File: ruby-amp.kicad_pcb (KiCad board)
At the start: 2 copper layers, 23 parts, among them J1 AudioJack3_Switch, J2 AudioJack2_Dual_Ground_Switch, P1 10k, P2 100K, P3 1k Lin, Q1 MPF102_DSG, U1 LM386

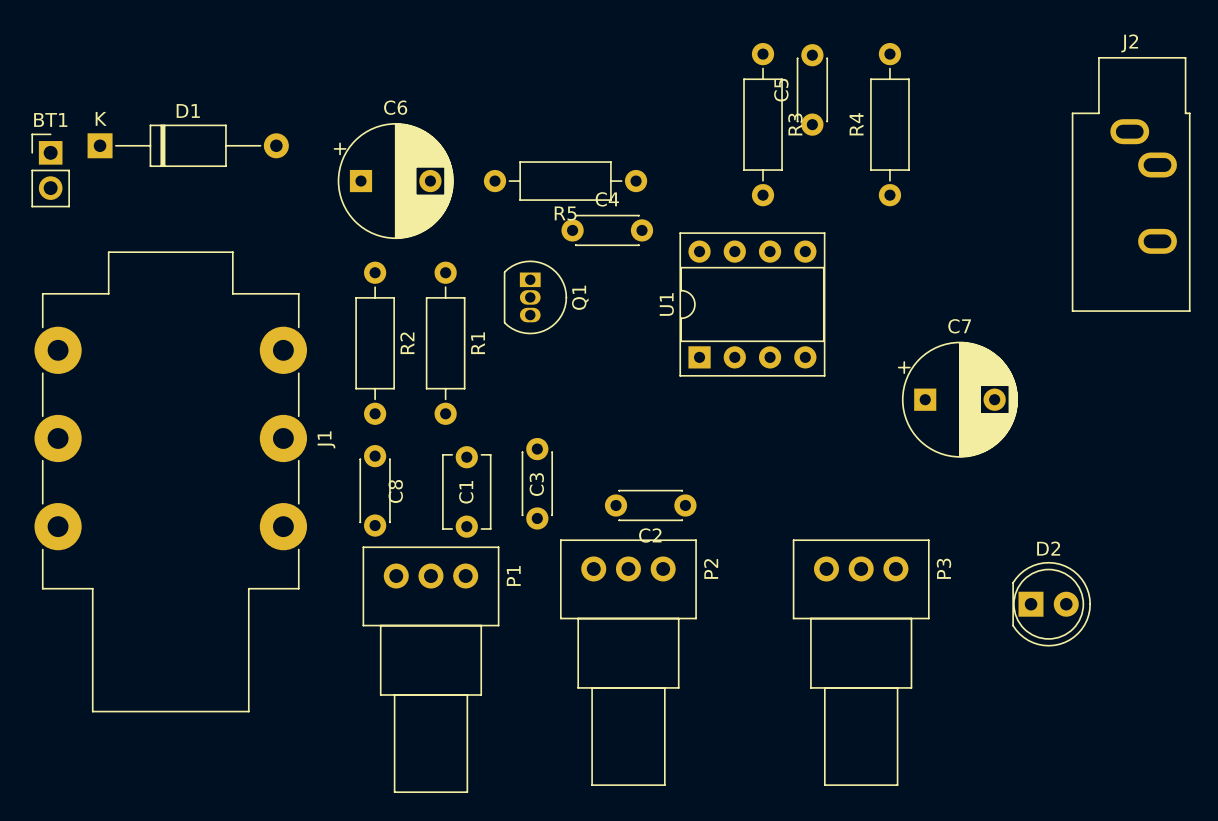
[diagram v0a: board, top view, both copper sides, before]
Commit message: PCB primera iteración
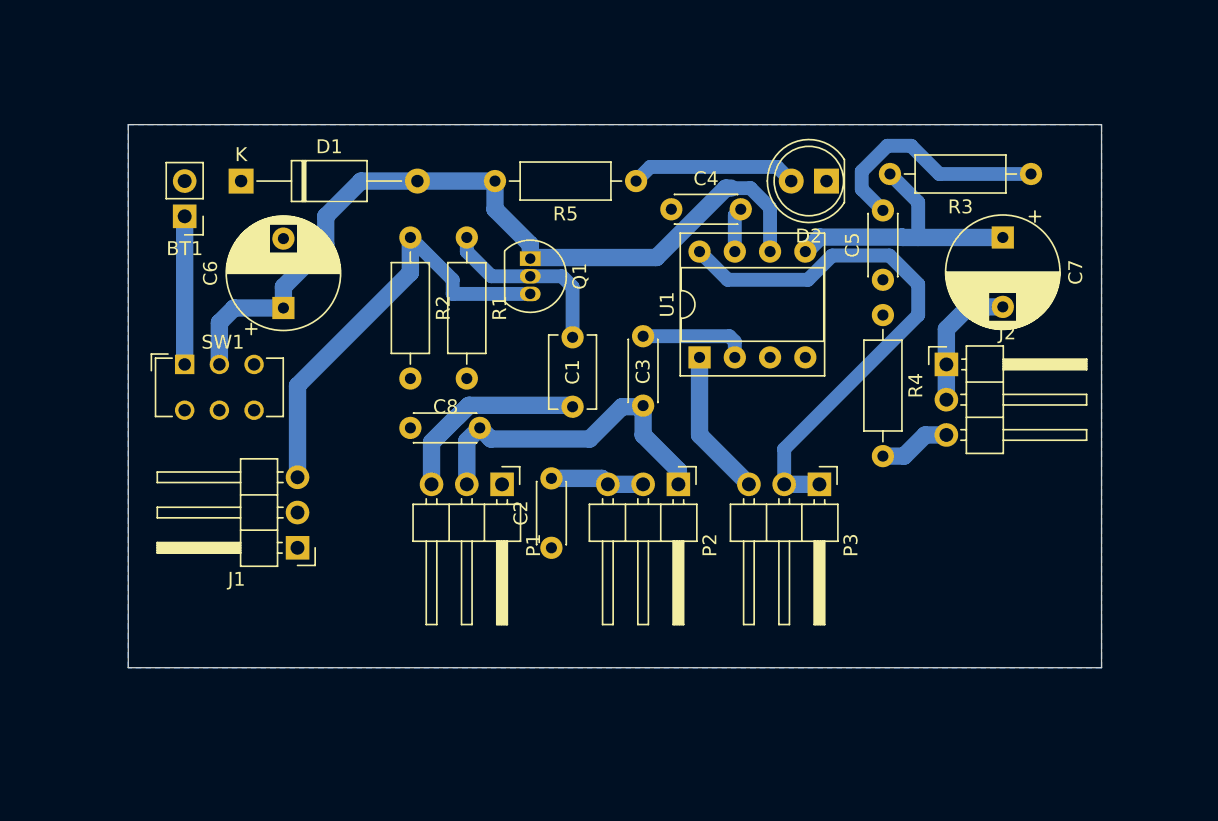
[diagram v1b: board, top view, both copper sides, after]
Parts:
- added SW1: SW_DPDT_x2, Button_Switch_THT:SW_CuK_JS202011CQN_DPDT_Straight, F.Cu at (111.3, 79.2)
- J1: value AudioJack3_Switch -> Input_Signal; footprint Connector_Audio:Jack_6.35mm_Neutrik_NMJ6HFD4_Horizontal -> Connector_PinHeader_2.54mm:PinHeader_1x03_P2.54mm_Horizontal
- J2: value AudioJack2_Dual_Ground_Switch -> Output_Signal; footprint Connector_Audio:Jack_3.5mm_CUI_SJ1-3533NG_Horizontal -> Connector_PinHeader_2.54mm:PinHeader_1x03_P2.54mm_Horizontal
- P1, P2, P3: footprint Potentiometer_THT:Potentiometer_Alps_RK09Y11_Single_Horizontal -> Connector_PinHeader_2.54mm:PinHeader_1x03_P2.54mm_Horizontal
- moved D2 33.9 mm to (157.5, 66.0), turned to 180 degrees
- moved J2 21.3 mm to (166.1, 79.2)
- moved R3 21.1 mm to (172.2, 65.5), turned to 180 degrees
- moved J1 14.3 mm to (119.4, 92.5), turned to 180 degrees
- moved C7 13.0 mm to (170.2, 70.1), turned to 270 degrees
- moved C5 12.3 mm to (161.5, 73.2)
- moved C1 11.5 mm to (139.2, 82.3)
- moved C3 11.1 mm to (144.3, 77.2)
- moved C6 10.7 mm to (118.4, 75.2), turned to 90 degrees
- moved BT1 10.7 mm to (111.3, 68.6), turned to 180 degrees
- moved D1 10.5 mm to (115.3, 66.0)
- moved C2 10.1 mm to (137.7, 92.5), turned to 90 degrees
- moved P1 10.1 mm to (134.1, 87.9)
- moved R4 8.65 mm to (161.5, 75.7), turned to 270 degrees
- moved P2 8.62 mm to (146.8, 87.9)
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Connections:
- BT1 pad 1: +9V -> Net-(BT1-Pad1)
- Q1 pad 3: Net-(J1-PadT) -> Net-(J1-Pad3)
- R2 pad 1: Net-(J1-PadT) -> Net-(J1-Pad3)
- R4 pad 2: Net-(J2-PadG) -> Net-(J2-Pad3)
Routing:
- net +9V: track 0.00 -> 58.3 mm
- net Net-(P3-Pad1): track 0.00 -> 39.1 mm
- net Net-(J1-Pad3): track 0.00 -> 31.6 mm
- net Net-(C3-Pad2): track 0.00 -> 24.3 mm
- net Net-(C7-Pad1): track 0.00 -> 20.1 mm
- net Net-(C1-Pad1): track 0.00 -> 18.1 mm
- net Net-(C5-Pad2): track 0.00 -> 17.2 mm
- net Net-(C1-Pad2): track 0.00 -> 13.3 mm
- net Net-(D2-Pad2): track 0.00 -> 12.0 mm
- net Net-(BT1-Pad1): track 0.00 -> 10.7 mm
- net Net-(P3-Pad3): track 0.00 -> 10.6 mm
- net Net-(C7-Pad2): track 0.00 -> 9.81 mm
- net Net-(C3-Pad1): track 0.00 -> 7.90 mm
- net Net-(C2-Pad2): track 0.00 -> 6.78 mm
- net Net-(J2-Pad3): track 0.00 -> 5.20 mm
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- added copper zone on B.Cu, net GNDREF
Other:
- board outline added: 70.1 x 39.1 mm
